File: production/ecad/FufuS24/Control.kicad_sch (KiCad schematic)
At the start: 25 parts, among them J2 Conn_01x02, U1 RP2040, U2 W25Q128JVS

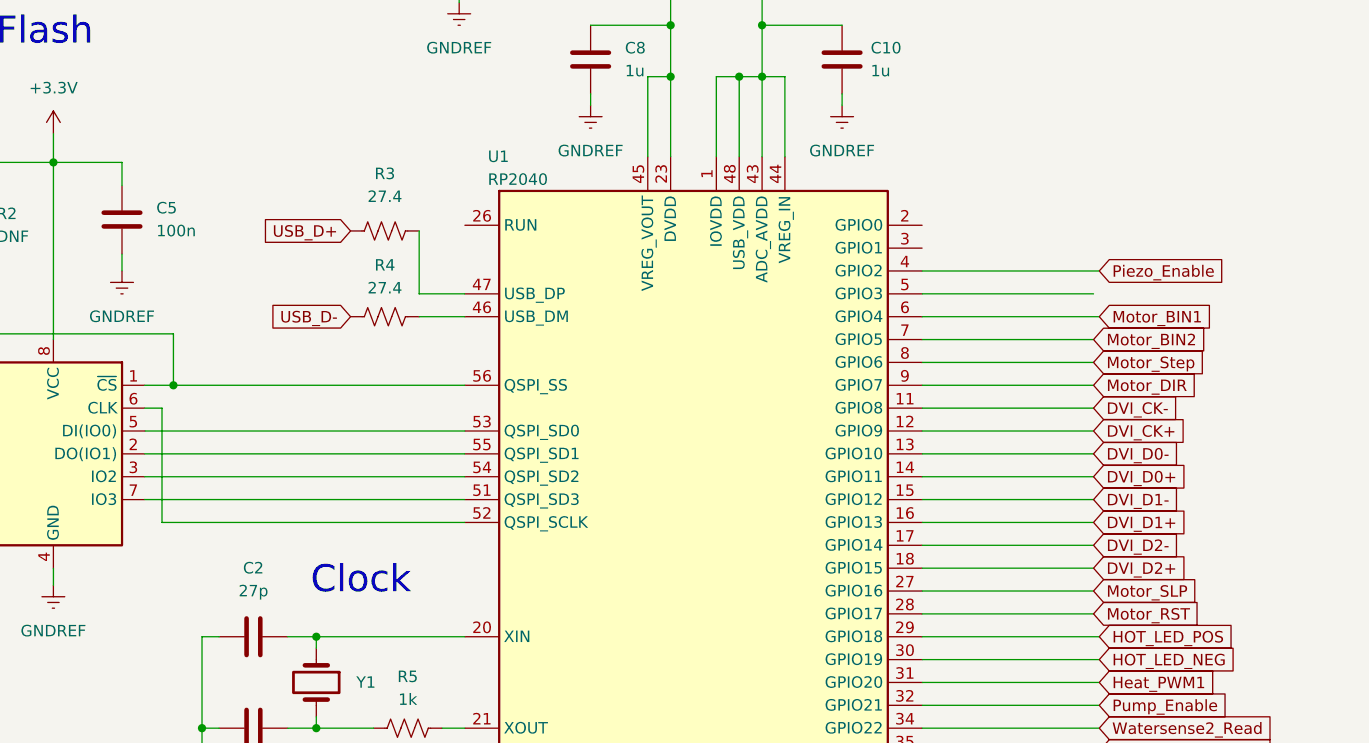
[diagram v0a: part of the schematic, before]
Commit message: HDMI + USB
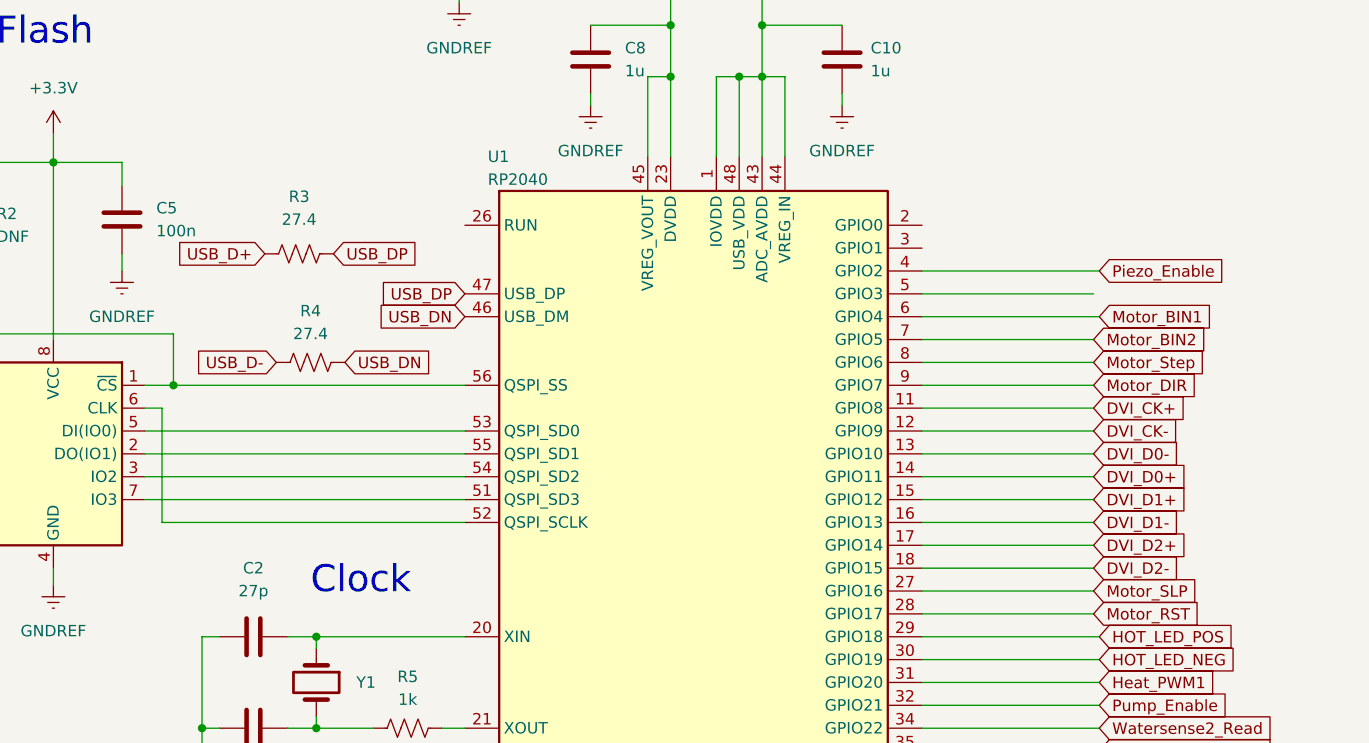
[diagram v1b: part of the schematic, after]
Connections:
- net DVI_CK+: now also U1.11 (GPIO8); no longer U1.12 (GPIO9)
- net DVI_CK-: now also U1.12 (GPIO9); no longer U1.11 (GPIO8)
- net DVI_D1+: now also U1.15 (GPIO12); no longer U1.16 (GPIO13)
- net DVI_D1-: now also U1.16 (GPIO13); no longer U1.15 (GPIO12)
- net DVI_D2+: now also U1.17 (GPIO14); no longer U1.18 (GPIO15)
- net DVI_D2-: now also U1.18 (GPIO15); no longer U1.17 (GPIO14)
- net USB_DP: now reaches R3.2, U1.47 (USB_DP)
- net USB_DN: now reaches R4.2, U1.46 (USB_DM)
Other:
- moved on the sheet: R3, R4
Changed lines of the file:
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@@
-    (stroke (width 0) (type default))
-  )
-  (wire (pts (xy 86.995 77.47) (xy 92.075 77.47))
     (stroke (width 0) (type default))
   )
@@
     (stroke (width 0) (type default))
   )
-  (wire (pts (xy 86.995 80.01) (xy 92.075 80.01))
-    (stroke (width 0) (type default))
-  )
   (wire (pts (xy 33.02 81.915) (xy 38.1 81.915))
     (stroke (width 0) (type default))
@@
   )
   (wire (pts (xy 125.095 47.625) (xy 125.095 53.34))
-    (stroke (width 0) (type default))
-  )
-  (wire (pts (xy 86.995 70.485) (xy 86.995 77.47))
     (stroke (width 0) (type default))
   )
@@
     )
   )
-  (global_label "USB_D-" (shape input) (at 79.375 80.01 180) (fields_autoplaced)
+  (global_label "USB_D-" (shape input) (at 71.12 85.09 180) (fields_autoplaced)
     (effects (font (size 1.27 1.27)) (justify right))
-    (property "Intersheetrefs" "${INTERSHEET_REFS}" (at 68.7698 80.01 0)
+    (property "Intersheetrefs" "${INTERSHEET_REFS}" (at 60.5148 85.09 0)
       (effects (font (size 1.27 1.27)) (justify right) hide)
     )
@@
     )
   )
-  (global_label "USB_D+" (shape input) (at 79.375 70.485 180) (fields_autoplaced)
+  (global_label "USB_D+" (shape input) (at 69.85 73.025 180) (fields_autoplaced)
     (effects (font (size 1.27 1.27)) (justify right))
-    (property "Intersheetrefs" "${INTERSHEET_REFS}" (at 68.7698 70.485 0)
+    (property "Intersheetrefs" "${INTERSHEET_REFS}" (at 59.2448 73.025 0)
       (effects (font (size 1.27 1.27)) (justify right) hide)
     )
   )
+  (global_label "USB_DN" (shape input) (at 92.075 80.01 180) (fields_autoplaced)
+    (effects (font (size 1.27 1.27)) (justify right))
+    (property "Intersheetrefs" "${INTERSHEET_REFS}" (at 81.7117 80.01 0)
+      (effects (font (size 1.27 1.27)) (justify right) hide)
+    )
+  )
   (global_label "Motor_SPI1_RX" (shape input) (at 161.925 130.81 0) (fields_autoplaced)
     (effects (font (size 1.27 1.27)) (justify left))
@@
     )
   )
+  (global_label "USB_DP" (shape input) (at 77.47 73.025 0) (fields_autoplaced)
+    (effects (font (size 1.27 1.27)) (justify left))
+    (property "Intersheetrefs" "${INTERSHEET_REFS}" (at 87.7728 73.025 0)
+      (effects (font (size 1.27 1.27)) (justify left) hide)
+    )
+  )
   (global_label "Motor_BIN1" (shape input) (at 162.56 80.01 0) (fields_autoplaced)
     (effects (font (size 1.27 1.27)) (justify left))
@@
     )
   )
+  (global_label "USB_DN" (shape input) (at 78.74 85.09 0) (fields_autoplaced)
+    (effects (font (size 1.27 1.27)) (justify left))
+    (property "Intersheetrefs" "${INTERSHEET_REFS}" (at 89.1033 85.09 0)
+      (effects (font (size 1.27 1.27)) (justify left) hide)
+    )
+  )
   (global_label "Motor_BIN2" (shape input) (at 161.925 82.55 0) (fields_autoplaced)
     (effects (font (size 1.27 1.27)) (justify left))
@@
     )
   )
-  (global_label "DVI_CK+" (shape input) (at 161.925 92.71 0) (fields_autoplaced)
+  (global_label "DVI_CK-" (shape input) (at 161.925 92.71 0) (fields_autoplaced)
     (effects (font (size 1.27 1.27)) (justify left))
     (property "Intersheetrefs" "${INTERSHEET_REFS}" (at 172.9536 92.71 0)
@@
     )
   )
-  (global_label "DVI_D1+" (shape input) (at 161.925 102.87 0) (fields_autoplaced)
+  (global_label "DVI_D1-" (shape input) (at 161.925 102.87 0) (fields_autoplaced)
     (effects (font (size 1.27 1.27)) (justify left))
     (property "Intersheetrefs" "${INTERSHEET_REFS}" (at 172.8931 102.87 0)
@@
     )
   )
-  (global_label "DVI_CK-" (shape input) (at 161.925 90.17 0) (fields_autoplaced)
+  (global_label "DVI_CK+" (shape input) (at 161.925 90.17 0) (fields_autoplaced)
     (effects (font (size 1.27 1.27)) (justify left))
     (property "Intersheetrefs" "${INTERSHEET_REFS}" (at 172.9536 90.17 0)
@@
     )
   )
-  (global_label "DVI_D2-" (shape input) (at 161.925 105.41 0) (fields_autoplaced)
+  (global_label "DVI_D2+" (shape input) (at 161.925 105.41 0) (fields_autoplaced)
     (effects (font (size 1.27 1.27)) (justify left))
     (property "Intersheetrefs" "${INTERSHEET_REFS}" (at 172.8931 105.41 0)
@@
     )
   )
-  (global_label "DVI_D1-" (shape input) (at 161.925 100.33 0) (fields_autoplaced)
+  (global_label "DVI_D1+" (shape input) (at 161.925 100.33 0) (fields_autoplaced)
     (effects (font (size 1.27 1.27)) (justify left))
     (property "Intersheetrefs" "${INTERSHEET_REFS}" (at 172.8931 100.33 0)
@@
     )
   )
-  (global_label "DVI_D2+" (shape input) (at 161.925 107.95 0) (fields_autoplaced)
+  (global_label "DVI_D2-" (shape input) (at 161.925 107.95 0) (fields_autoplaced)
     (effects (font (size 1.27 1.27)) (justify left))
     (property "Intersheetrefs" "${INTERSHEET_REFS}" (at 172.8931 107.95 0)
@@
     (property "Intersheetrefs" "${INTERSHEET_REFS}" (at 182.9622 125.73 0)
       (effects (font (size 1.27 1.27)) (justify left) hide)
+    )
+  )
+  (global_label "USB_DP" (shape input) (at 92.075 77.47 180) (fields_autoplaced)
+    (effects (font (size 1.27 1.27)) (justify right))
+    (property "Intersheetrefs" "${INTERSHEET_REFS}" (at 81.7722 77.47 0)
+      (effects (font (size 1.27 1.27)) (justify right) hide)
     )
   )
@@
     )
   )
-  (symbol (lib_id "Device:R_US") (at 83.185 70.485 90) (unit 1)
-    (in_bom yes) (on_board yes) (dnp no) (fields_autoplaced)
-    (property "Reference" "R3" (at 83.185 64.135 90)
-      (effects (font (size 1.27 1.27)))
-    )
-    (property "Value" "27.4" (at 83.185 66.675 90)
-      (effects (font (size 1.27 1.27)))
-    )
-    (property "Footprint" "footprints:RESC2012X60N" (at 83.439 69.469 90)
-      (effects (font (size 1.27 1.27)) hide)
-    )
-    (property "Datasheet" "~" (at 83.185 70.485 0)
+  (symbol (lib_id "Device:R_US") (at 73.66 73.025 90) (unit 1)
+    (in_bom yes) (on_board yes) (dnp no) (fields_autoplaced)
+    (property "Reference" "R3" (at 73.66 66.675 90)
+      (effects (font (size 1.27 1.27)))
+    )
+    (property "Value" "27.4" (at 73.66 69.215 90)
+      (effects (font (size 1.27 1.27)))
+    )
+    (property "Footprint" "footprints:RESC2012X60N" (at 73.914 72.009 90)
+      (effects (font (size 1.27 1.27)) hide)
+    )
+    (property "Datasheet" "~" (at 73.66 73.025 0)
       (effects (font (size 1.27 1.27)) hide)
     )
@@
     )
   )
-  (symbol (lib_id "Device:R_US") (at 83.185 80.01 90) (unit 1)
-    (in_bom yes) (on_board yes) (dnp no) (fields_autoplaced)
-    (property "Reference" "R4" (at 83.185 74.295 90)
-      (effects (font (size 1.27 1.27)))
-    )
-    (property "Value" "27.4" (at 83.185 76.835 90)
-      (effects (font (size 1.27 1.27)))
-    )
-    (property "Footprint" "footprints:RESC2012X60N" (at 83.439 78.994 90)
-      (effects (font (size 1.27 1.27)) hide)
-    )
-    (property "Datasheet" "~" (at 83.185 80.01 0)
-      (effects (font (size 1.27 1.27)) hide)
-    )
+  (symbol (lib_id "Device:R_US") (at 74.93 85.09 90) (unit 1)
+    (in_bom yes) (on_board yes) (dnp no) (fields_autoplaced)
+    (property "Reference" "R4" (at 74.93 79.375 90)
+      (effects (font (size 1.27 1.27)))
+    )
+    (property "Value" "27.4" (at 74.93 81.915 90)
+      (effects (font (size 1.27 1.27)))
+    )
+    (property "Footprint" "footprints:RESC2012X60N" (at 75.184 84.074 90)
+      (effects (font (size 1.27 1.27)) hide)
+    )
+    (property "Datasheet" "~" (at 74.93 85.09 0)
+      (effects (font (size 1.27 1.27)) hide)
+    )

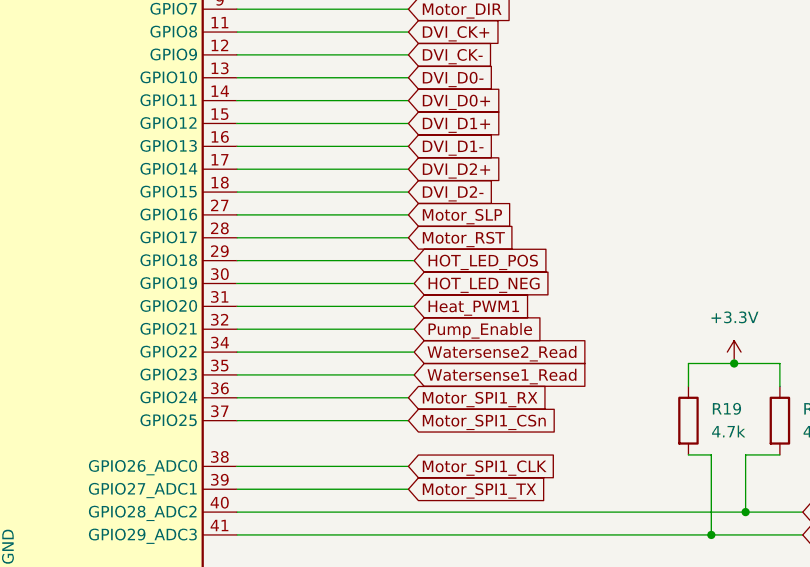
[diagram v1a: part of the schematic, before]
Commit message: review changes
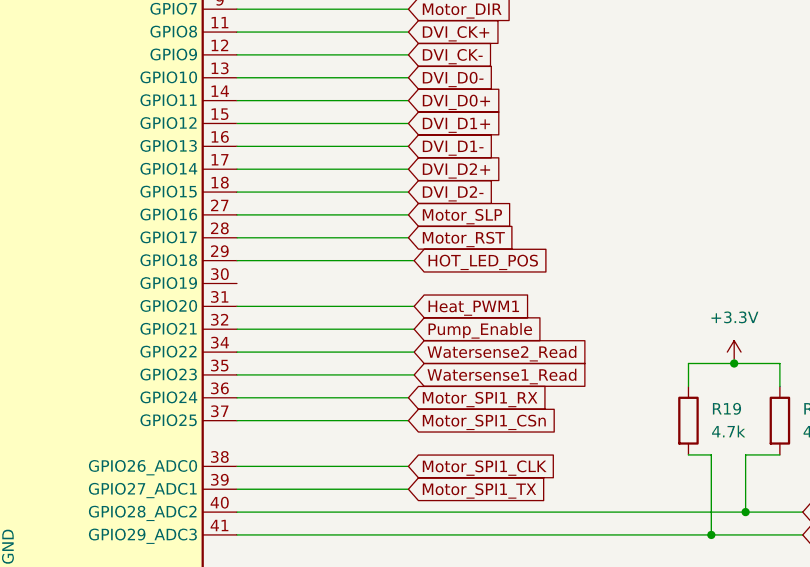
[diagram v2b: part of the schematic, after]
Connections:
- net HOT_LED_NEG: no longer names the net of U1.30 (GPIO19)
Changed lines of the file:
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@@
-    (stroke (width 0) (type default))
-  )
-  (wire (pts (xy 142.875 118.11) (xy 162.56 118.11))
     (stroke (width 0) (type default))
   )
@@
       (effects (font (size 1.27 1.27)) (justify left) hide)
     )
-  )
-  (global_label "HOT_LED_NEG" (shape input) (at 162.56 118.11 0) (fields_autoplaced)
-    (effects (font (size 1.27 1.27)) (justify left))
-    (property "Intersheetrefs" "${INTERSHEET_REFS}" (at 178.3056 118.11 0)
-      (effects (font (size 1.27 1.27)) (justify left) hide)
-    )

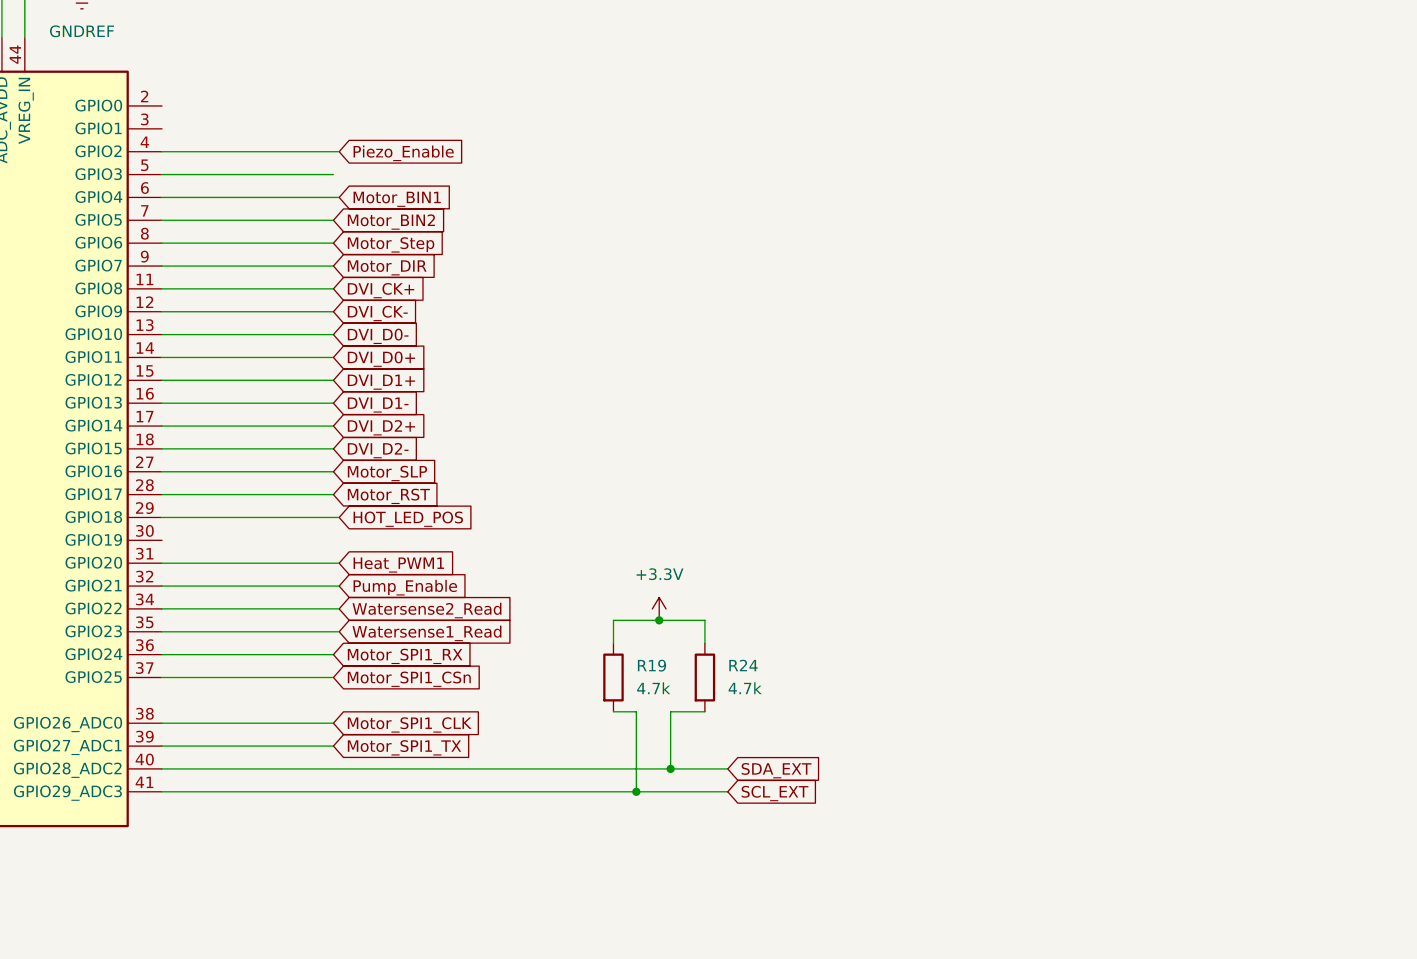
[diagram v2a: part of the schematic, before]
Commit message: i am pulling my hair out
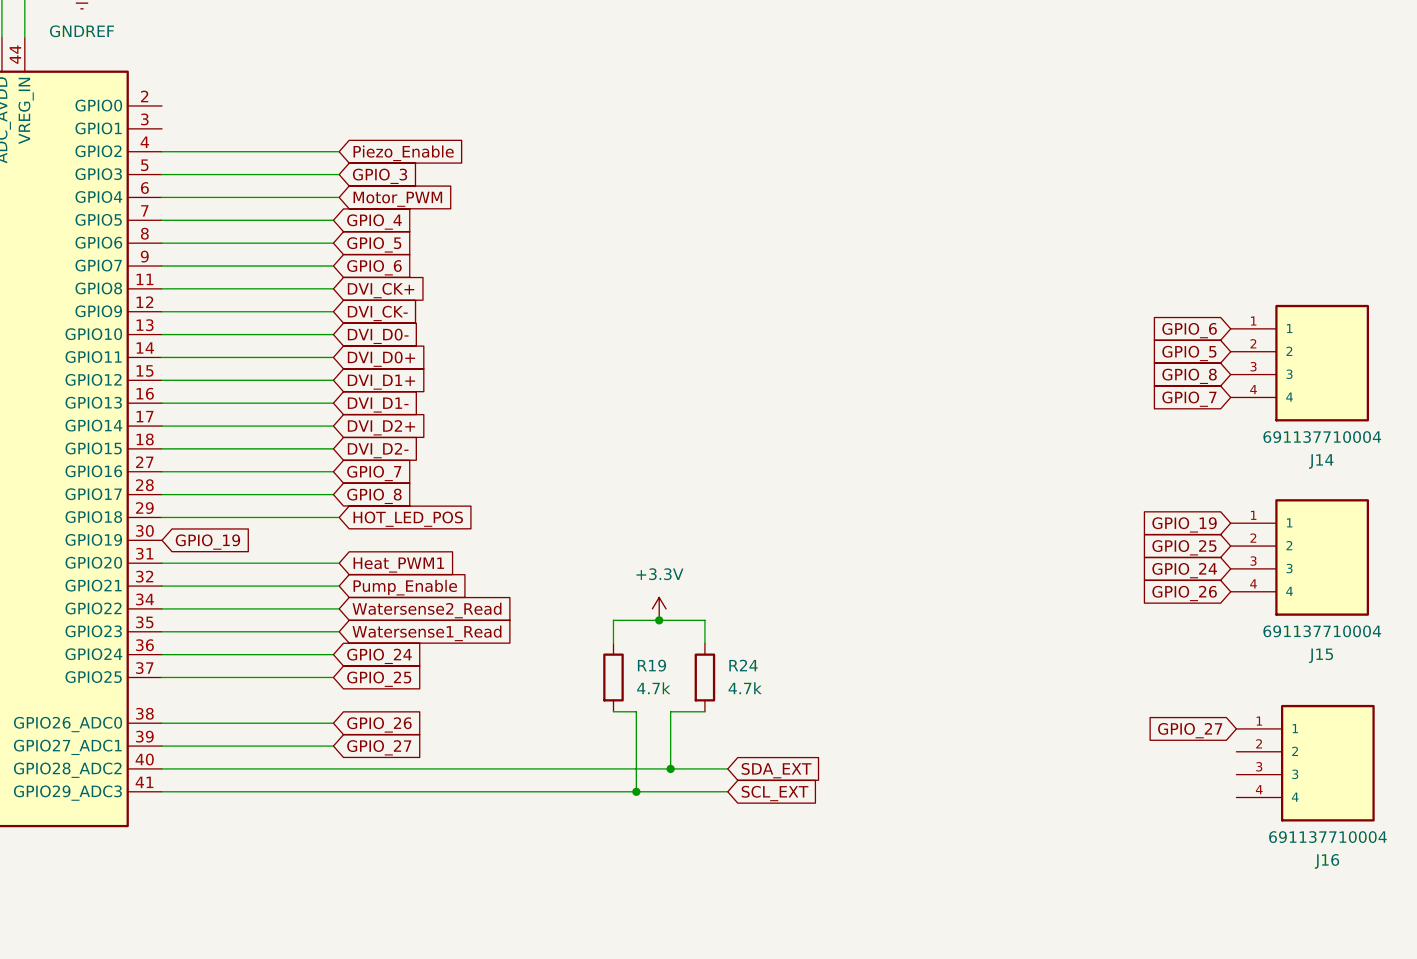
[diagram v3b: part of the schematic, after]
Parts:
- added J14, J15, J16: 691137710004, footprints:PWR_4POS, symbol PWR_4POS:691137710004
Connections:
- net GPIO_19: now reaches U1.30 (GPIO19)
- net GPIO_19: now also J15.1
- net GPIO_3: now reaches U1.5 (GPIO3)
- net Motor_BIN1 renamed Motor_PWM
- net Motor_BIN2 renamed GPIO_4
- net Motor_DIR renamed GPIO_6
- net GPIO_6: now also J14.1
- net Motor_RST renamed GPIO_8
- net GPIO_8: now also J14.3
- net Motor_SLP renamed GPIO_7
- net GPIO_7: now also J14.4
- net Motor_SPI1_CLK renamed GPIO_26
- net GPIO_26: now also J15.4
- net Motor_SPI1_CSn renamed GPIO_25
- net GPIO_25: now also J15.2
- net Motor_SPI1_RX renamed GPIO_24
- net GPIO_24: now also J15.3
- net Motor_SPI1_TX renamed GPIO_27
- net GPIO_27: now also J16.1
- net Motor_Step renamed GPIO_5
- net GPIO_5: now also J14.2
